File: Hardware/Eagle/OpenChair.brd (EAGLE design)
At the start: 80 x 50 mm, 89 parts, among them IC1 7805DT, IC2 AP2112K-3.3TRG1 3.3V, Q1 12MHz 3.2x2.5, Q2 BSS84, Q3 BSS84, Q4 16MHz 3.2x2.5, SW1 RESET, U1 RJ45-8PTH, U2 NXP_LPC1768_FBD100, U3 LMC7101AIM5, U4 NRF_8001_R2Q32_T, Y1 ABS25, Y2 ABS25-32.768kHz

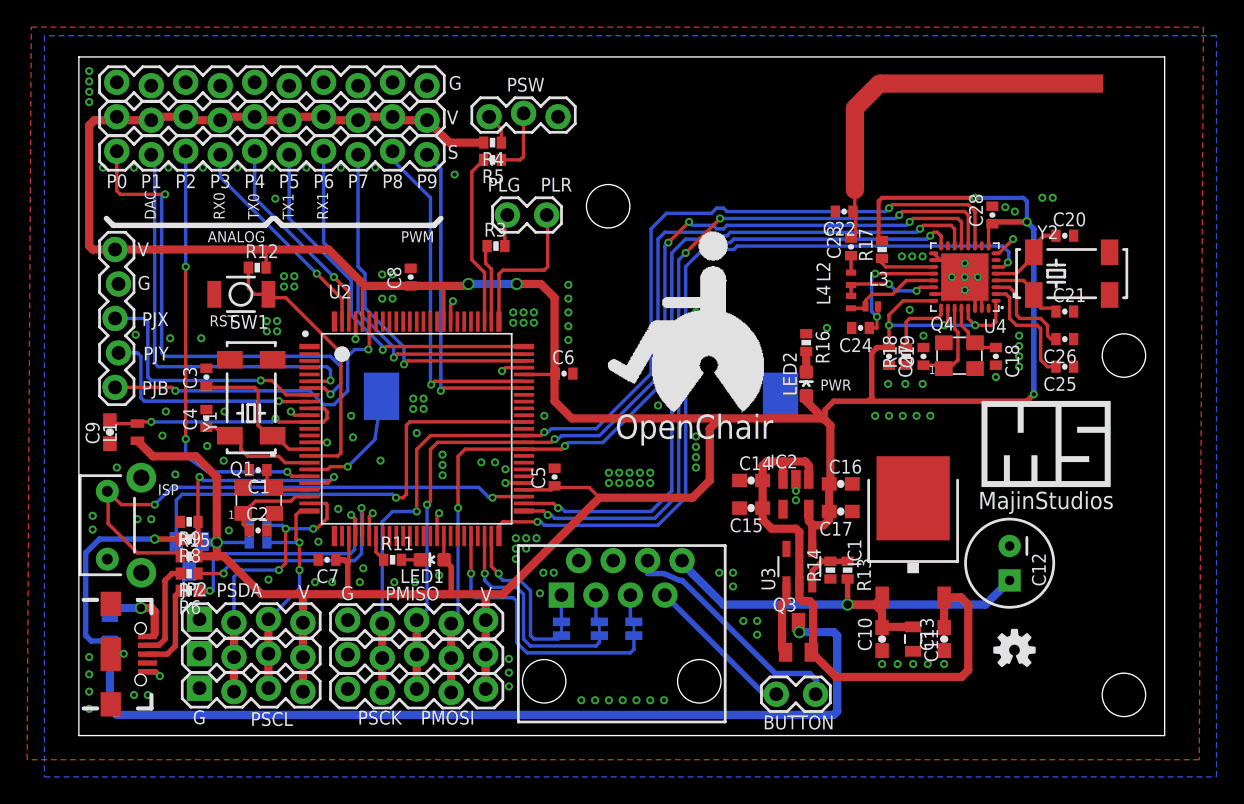
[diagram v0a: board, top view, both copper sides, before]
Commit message: Added Gerber RS274X files and updated PDF
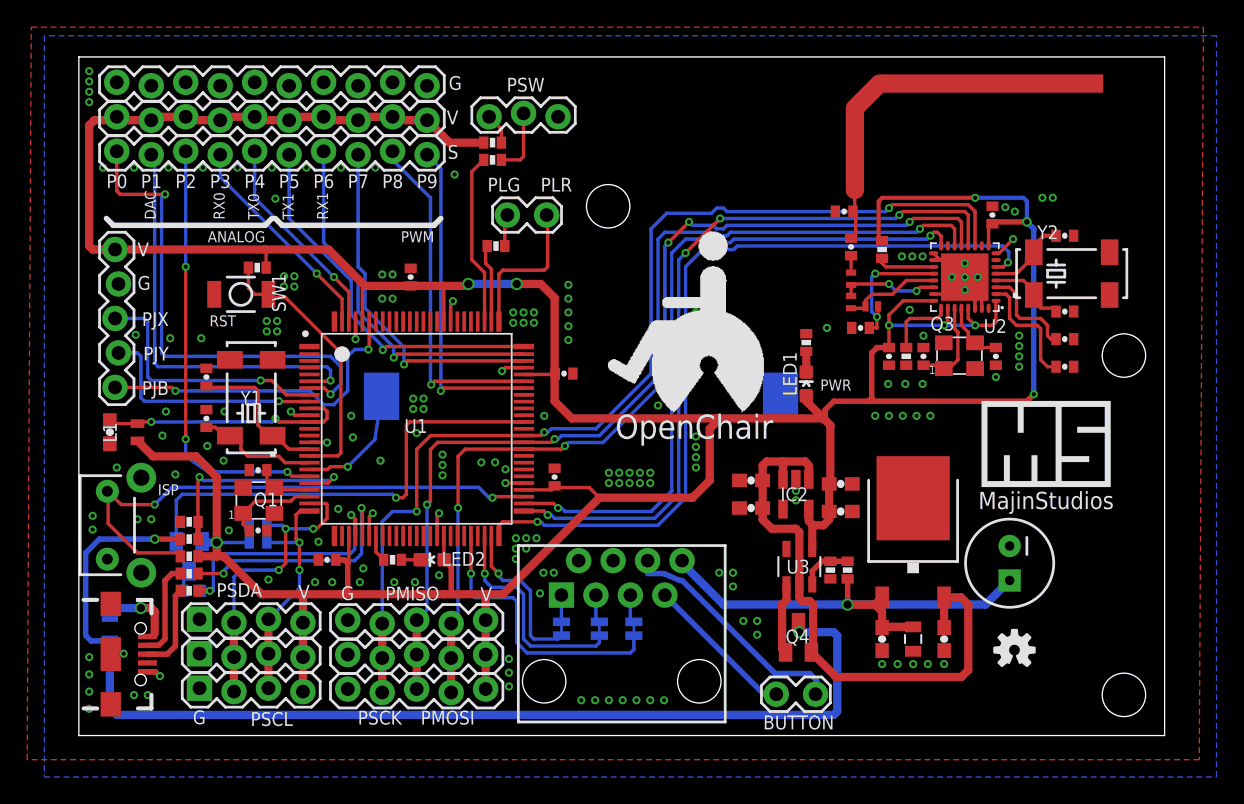
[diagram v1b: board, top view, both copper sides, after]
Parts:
- C1, C2: value 18pF -> 1uF; device SparkFun-Passives:0402-CAP -> SparkFun-Passives:0603-CAP
- C10: value 1uF -> 12pF; device SparkFun-Passives:0603-CAP -> SparkFun-Passives:0402-CAP
- C11: value 0.33uF -> 12pF; device SparkFun-Passives:0805 -> SparkFun-Passives:0402-CAP
- C12: value 220uF 25V -> 18pF; device SparkFun-Capacitors:CPOL-RADIAL-100UF-25V -> SparkFun-Passives:0402-CAP
- C13: value 1uF -> 18pF; device SparkFun-Passives:0603-CAP -> SparkFun-Passives:0402-CAP
- C14, C9: value 1uF -> 0.1uF; device SparkFun-Passives:0603-CAP -> SparkFun-Passives:0402-CAP
- C15, C16: value 10uF 10V -> 0.1uF; device SparkFun-Passives:0603-CAP -> SparkFun-Passives:0402-CAP
- C18: value 18pF -> 1.2pF
- C19: value 18pF -> 1.8pF
- C20: value 12pF -> 2.2nF
- C22: value 1.2pF -> 12pF
- C23: value 1.8pF -> 18pF
- C24: value 2.2nF -> 18pF
- C25: value 100nF -> 0.1uF
- C26: value 33nF -> 100nF
- C28: value 0.1uF -> 33nF
- C3: value 12pF -> 10uF 10V; device SparkFun-Passives:0402-CAP -> SparkFun-Passives:0603-CAP
- C4: value 12pF -> 0.33uF; device SparkFun-Passives:0402-CAP -> SparkFun-Passives:0805
- C5: value 0.1uF -> 220uF 25V; device SparkFun-Passives:0402-CAP -> SparkFun-Capacitors:CPOL-RADIAL-100UF-25V
- C6: value 0.1uF -> 10uF 10V; device SparkFun-Passives:0402-CAP -> SparkFun-Passives:0603-CAP
- C7, C8: value 0.1uF -> 1uF; device SparkFun-Passives:0402-CAP -> SparkFun-Passives:0603-CAP
- JP1: value (none) -> M10LOCK; device SparkFun-Connectors:1X05_LOCK -> SparkFun-Connectors:1X10_LOCK
- JP10: value USB_MICROB_PLUGCONN-11752 -> (none); device SparkFun-Connectors:USB-B-MICRO-SMD_V03 -> SparkFun-Connectors:1X05_LOCK
- JP11: value M10LOCK -> (none); device SparkFun-Connectors:1X10_LOCK -> SparkFun-Connectors:1X03_LOCK
- JP12: value (none) -> USB_MICROB_PLUGCONN-11752; device SparkFun-Connectors:1X03_LOCK -> SparkFun-Connectors:USB-B-MICRO-SMD_V03
- JP13: value (none) -> M02LOCK; device SparkFun-Connectors:1X05_LOCK -> SparkFun-Connectors:1X02_LOCK
- JP2: device SparkFun-Connectors:1X04_LOCK -> SparkFun-Connectors:1X05_LOCK
- JP3: device SparkFun-Connectors:1X05_LOCK -> SparkFun-Connectors:1X04_LOCK
- JP4: value (none) -> M10LOCK; device SparkFun-Connectors:1X04_LOCK -> SparkFun-Connectors:1X10_LOCK
- JP7: value M02LOCK -> M10LOCK; device SparkFun-Connectors:1X02_LOCK -> SparkFun-Connectors:1X10_LOCK
- JP8: value M10LOCK -> (none); device SparkFun-Connectors:1X10_LOCK -> SparkFun-Connectors:1X05_LOCK
- JP9: value M10LOCK -> (none); device SparkFun-Connectors:1X10_LOCK -> SparkFun-Connectors:1X04_LOCK
- Q3: value BSS84 -> 16MHz 3.2x2.5; device transistor-small-signal:SOT23 -> GHI:CRYSTAL_3.2X2.5
- Q4: value 16MHz 3.2x2.5 -> BSS84; device GHI:CRYSTAL_3.2X2.5 -> transistor-small-signal:SOT23
- R1: value 4.7k -> 470
- R10: value 1.5K -> 10k
- R11: value 470 -> 22k
- R14, R15: value 10k -> 4.7k
- R16: value 470 -> 10k
- R18: value 22k -> 470
- R2: value 4.7k -> 10k
- R3: value 330 -> 10k
- R4, R5: value 10k -> 33
- R6: value 33 -> 100k
- R7: value 33 -> 1k
- R8: value 1k -> 1.5K
- R9: value 100k -> 470
- U1: value RJ45-8PTH -> NXP_LPC1768_FBD100; device SparkFun-Connectors:RJ45-8 -> alvaroferran:QFP50P1600X1600X160-100N
- U2: value NXP_LPC1768_FBD100 -> NRF_8001_R2Q32_T; device alvaroferran:QFP50P1600X1600X160-100N -> alvaroferran:QFN50P500X500X90-33N
- U4: value NRF_8001_R2Q32_T -> RJ45-8PTH; device alvaroferran:QFN50P500X500X90-33N -> SparkFun-Connectors:RJ45-8
- moved R10 56.7 mm to (59.2, 35.8), flipped to the top, turned to 90 degrees
- moved C11 55.5 mm to (9.40, 26.4), turned to 90 degrees
- moved C12 55.4 mm to (13.2, 15.1), turned to 0 degrees
- moved C4 54.5 mm to (61.5, 7.11), turned to 270 degrees
- moved C17 54.2 mm to (2.29, 22.4), turned to 90 degrees
- moved JP13 53.8 mm to (51.6, 3.05), turned to 0 degrees
- moved C10 52.4 mm to (9.40, 23.4)
- moved C13 52.1 mm to (13.2, 19.6), turned to 180 degrees
- moved JP12 51.6 mm to (2.35, 6.00), turned to 0 degrees
- moved R12 47.7 mm to (55.4, 12.2), turned to 90 degrees
- moved C2 46.7 mm to (59.2, 7.11), turned to 90 degrees
- moved C7 45.8 mm to (63.8, 7.11), turned to 90 degrees
- moved JP8 45.5 mm to (19.8, 3.30)
- moved JP9 45.1 mm to (8.89, 3.37)
- moved R1 43.0 mm to (53.6, 29.0), flipped to the top, turned to 270 degrees
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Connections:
- net !RST: now also R2.1, U1.17; no longer R12.1, U2.17
- net 3.3V: now also C14.1, C15.1, C25.1, C8.2, C9.1, JP1.1, JP1.10, JP1.2, JP1.3, JP1.4, JP1.6, JP1.7, JP1.8, JP1.9, JP10.5, JP2.5, JP3.4, JP9.4, R10.2, R14.1, R15.1, R2.2, R3.2, U1.28, U1.42, U1.54, U1.71, U1.84, U1.96, U2.1, U2.24, U2.26, U2.29, U2.9; no longer C17.2, C28.1, C5.1, C7.1, C8.1, JP13.5, JP2.4, JP3.5, JP4.4, JP8.1, JP8.10, JP8.2, JP8.3, JP8.4, JP8.6, JP8.7, JP8.8, JP8.9, R1.1, R12.2, R15.2, R2.1, R4.2, U2.28, U2.42, U2.54, U2.71, U2.84, U2.96, U4.1, U4.24, U4.26, U4.29, U4.9
- net 5V: now also C1.2, C3.1, C7.2, Q4.2; no longer C13.2, C14.2, C15.1, Q3.2
- net BTNA: now also JP13.2, U4.6; no longer JP14.2, U1.6
- net BTNB: now also JP13.1, U4.7; no longer JP14.1, U1.7
- net D+: now also JP12.D+1, R5.2; no longer JP10.D+1, R6.2
- net D-: now also JP12.D-1, R4.2; no longer JP10.D-1, R7.2
- net DCC: now also U2.32; no longer U4.32
- net GND: now also C1.1, C10.2, C13.2, C14.2, C2.1, C23.2, C25.2, C28.1, C7.1, C8.1, C9.2, JP10.4, JP11.1, JP12.GND1, JP12.SHIELD1, JP12.SHIELD2, JP12.SHIELD3, JP4.10, JP4.2, JP4.3, JP4.4, JP4.5, JP4.6, JP4.7, JP4.8, JP4.9, JP8.1, R1.1, R11.1, R12.1, R6.2, U1.11, U1.15, U1.31, U1.41, U1.55, U1.72, U1.83, U1.97, U2.17, U2.18, U2.23, U2.30, U2.33, U2.8, U4.2, U4.4; no longer C1.2, C10.1, C13.1, C14.1, C19.2, C2.2, C25.1, C28.2, C7.2, C8.2, C9.1, JP1.1, JP10.GND1, JP10.SHIELD1, JP10.SHIELD2, JP10.SHIELD3, JP12.1, JP13.4, JP9.10, JP9.2, JP9.3, JP9.4, JP9.5, JP9.6, JP9.7, JP9.8, JP9.9, R14.1, R16.1, R18.1, R9.2, U1.2, U1.4, U2.11, U2.15, U2.41, U2.55, U2.72, U2.83, U2.97, U4.17, U4.18, U4.23, U4.30, U4.31, U4.33, U4.8
- net ISP: now also R3.1, U1.53; no longer R15.1, U2.53
- net N$1: now also JP14.2, R18.2; no longer JP7.2, R3.2
- net N$11: now also JP11.3, R17.1; no longer JP12.3, R4.1
- net N$12: now also R6.1, R7.1, U1.21; no longer R8.1, R9.1, U2.21
- net N$13: now also R5.1, R8.2, U1.29; no longer R10.2, R6.1, U2.29
- net N$14: now also R9.1, U1.32; no longer R11.1, U2.32
- net N$15: now also LED2.C, R9.2; no longer LED1.C, R11.2
- net N$16: now also R4.1, U1.30; no longer R7.1, U2.30
- net N$17: now also R8.1; no longer R10.1
- net N$18: now also Q4.1; no longer Q3.1
- net N$2: now also SJ3.1, U4.1; no longer SJ1.1, U1.1
- net N$20: now also R12.2; no longer R14.2
- net N$21: now also R11.2, U2.25; no longer R18.2, U4.25
- net N$22: now also C26.2, U2.2; no longer C25.2, U4.2
- net N$23: now also C28.2, U2.3; no longer C26.2, U4.3
- net N$24: now also R10.1, U2.19; no longer R17.1, U4.19
- net N$25: now also U2.22; no longer U4.22
- net N$26: now also U2.21; no longer U4.21
- net N$29: now also C19.1; no longer C23.1
- net N$3: now also U4.3; no longer U1.3
- net N$30: now also C18.1, C19.2; no longer C22.1, C23.2
- net N$4: now also SJ1.1, U4.5; no longer SJ3.1, U1.5
- net N$5: now also JP12.VBUS1; no longer JP10.VBUS1
- net N$6: now also JP11.2, R16.1; no longer JP12.2, R5.1
- net N$7: now also LED1.C, R1.2; no longer LED2.C, R16.2
- net P0: now also JP7.1, U1.7; no longer JP11.1, U2.7
- net P1: now also JP7.2, U1.6; no longer JP11.2, U2.6
- net P2: now also JP7.3, U1.20; no longer JP11.3, U2.20
- net P3: now also JP7.4, U1.99; no longer JP11.4, U2.99
- net P4: now also JP7.5, U1.98; no longer JP11.5, U2.98
- net P5: now also JP7.6, U1.75; no longer JP11.6, U2.75
- net P6: now also JP7.7, U1.74; no longer JP11.7, U2.74
- net P7: now also JP7.8, U1.73; no longer JP11.8, U2.73
- net P8: now also JP7.9, U1.70; no longer JP11.9, U2.70
- net P9: now also JP7.10, U1.69; no longer JP11.10, U2.69
- net PACT: now also U1.50, U2.6; no longer U2.50, U4.6
- net PJB: now also JP10.1, U1.95; no longer JP13.1, U2.95
- net PJX: now also JP10.3, U1.8; no longer JP13.3, U2.8
- net PJY: now also JP10.2, U1.9; no longer JP13.2, U2.9
- net PLG: now also R18.1, U1.77; no longer R3.1, U2.77
- net PLR: now also JP14.1, U1.76; no longer JP7.1, U2.76
- net PMISO: now also JP2.3, JP8.3, U1.61, U2.14; no longer JP1.3, JP3.3, U2.61, U4.14
- net PMOSI: now also JP2.4, JP8.4, U1.60, U2.13; no longer JP1.4, JP3.4, U2.60, U4.13
- net PRDY: now also U1.52, U2.16; no longer U2.52, U4.16
- net PREQ: now also U1.51, U2.12; no longer U2.51, U4.12
- net PSCK: now also JP2.2, JP8.2, U1.62, U2.11; no longer JP1.2, JP3.2, U2.62, U4.11
- net PSCL: now also JP3.2, JP9.2, R15.2, U1.24; no longer JP2.2, JP4.2, R2.2, U2.24
- net PSDA: now also JP3.3, JP9.3, R14.2, U1.25; no longer JP2.3, JP4.3, R1.2, U2.25
- net PSW: now also R16.2, U1.78; no longer R5.2, U2.78
- net RX2: now also SJ3.2, U1.49; no longer SJ1.2, U2.49
- net RX3: now also U1.47; no longer U2.47
- net RXT1: now also C11.1, U1.16; no longer C3.1, U2.16
- net RXT2: now also C10.1, U1.18; no longer C4.1, U2.18
- net TX2: now also U1.48; no longer U2.48
- net TX3: now also SJ1.2, U1.46; no longer SJ3.2, U2.46
- net USBC: now also U1.64; no longer U2.64
- net VBAT: now also U1.19; no longer U2.19
- net VCC: now also Q4.3, R7.2; no longer Q3.3, R8.2
- net VDDA: now also C17.2, U1.10, U1.12; no longer C9.2, U2.10, U2.12
- net VDD_PA: now also C20.1, U2.20; no longer C24.1, U4.20
- net VIN: now also C2.2, C4.1, C5.1, U4.8; no longer C10.2, C11.1, C12.1, U1.8
- net XC1: now also C24.1, Q3.3, U2.28; no longer C18.1, Q4.3, U4.28
- net XC2: now also C23.1, Q3.1, U2.27; no longer C19.1, Q4.1, U4.27
- net XL1: now also C22.1, U2.5; no longer C20.1, U4.5
- net XL2: now also U2.4; no longer U4.4
- net XT1: now also C13.1, U1.22; no longer C1.1, U2.22
- net XT2: now also C12.1, U1.23; no longer C2.1, U2.23
